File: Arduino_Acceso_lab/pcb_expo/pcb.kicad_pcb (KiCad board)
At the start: 2 copper layers, 88.4 x 55.4 mm, 15 parts, among them P1 modulo wifi, P20 CONN_01X02, U1 LM2576

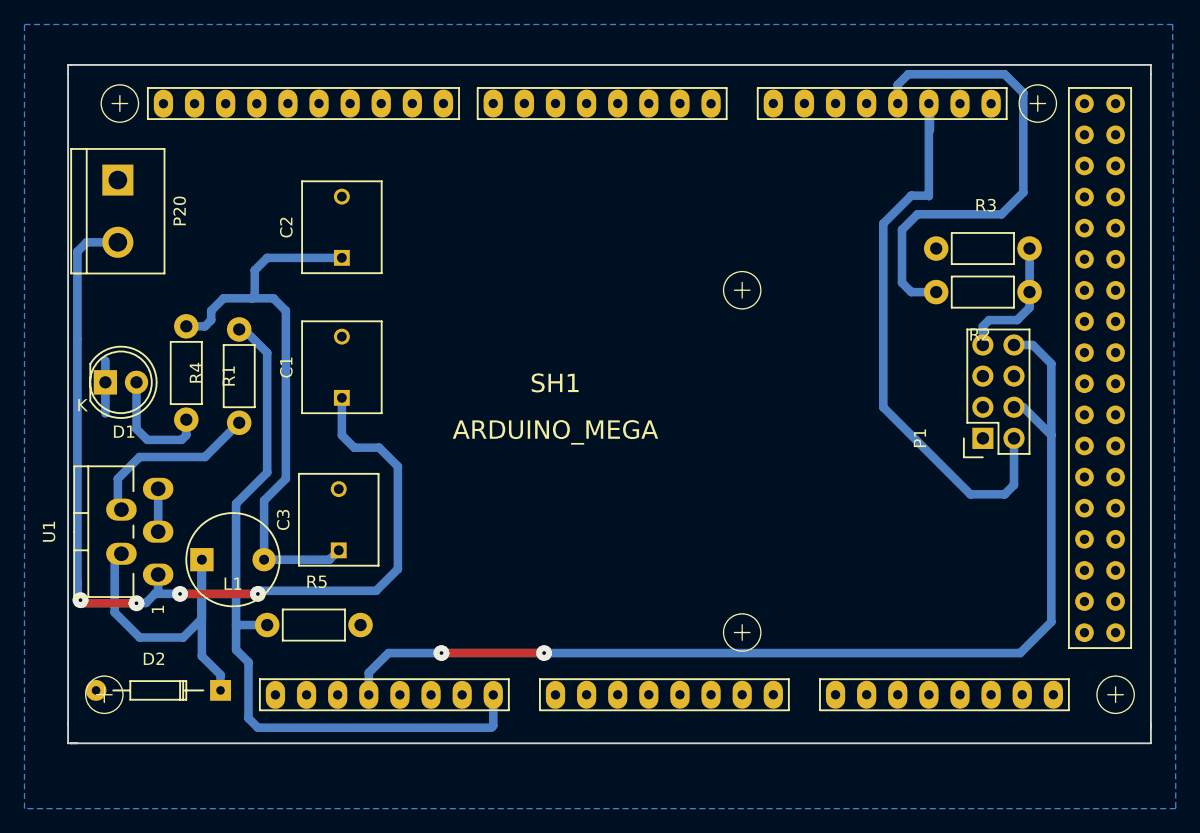
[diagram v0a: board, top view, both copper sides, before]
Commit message: Versión corregida por DJB del Shield Wifi para Arduini Mega.
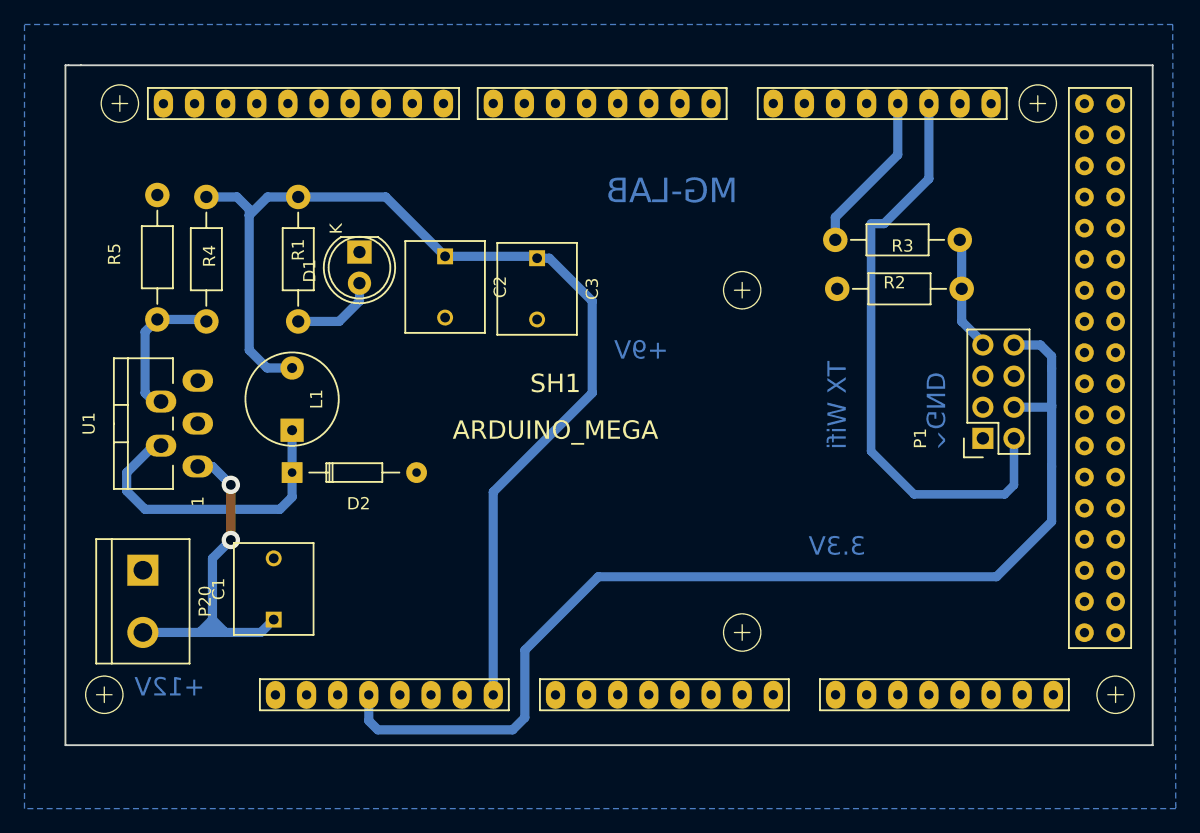
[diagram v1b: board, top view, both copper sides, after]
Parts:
- R1, R2, R3, R4, R5: footprint Resistors_ThroughHole:Resistor_Horizontal_RM7mm -> Resistors_ThroughHole:Resistor_Horizontal_RM10mm
- moved P20 31.9 mm to (114.8, 121.5)
- moved C3 28.8 mm to (147.0, 93.5), turned to 270 degrees
- moved R5 26.5 mm to (116.0, 98.5), turned to 90 degrees
- moved D1 23.3 mm to (132.5, 93.0), turned to 270 degrees
- moved C1 18.9 mm to (125.5, 123.0)
- moved D2 18.7 mm to (127.0, 111.0), turned to 0 degrees
- moved R4 18.6 mm to (120.0, 88.5), turned to 270 degrees
- moved L1 14.0 mm to (127.0, 105.0), turned to 90 degrees
- moved R1 14.0 mm to (127.5, 88.5)
- moved U1 9.40 mm to (115.5, 107.0)
- moved R3 8.72 mm to (171.5, 96.0)
- moved C2 8.43 mm to (139.5, 93.3), turned to 270 degrees
- moved R2 7.12 mm to (181.5, 92.0)
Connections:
- net /3.3 renamed +3.3VP
- C2 pad 1: Net-(C2-Pad1) -> +9V
- C3 pad 1: Net-(C2-Pad1) -> +9V
- L1 pad 2: Net-(C2-Pad1) -> +9V
- P1 pad 2: /RXwifi -> /TXwifi2
- R1 pad 1: Net-(C2-Pad1) -> +9V
- R2 pad 2: /TXwifi -> /RXwifi
- R4 pad 1: Net-(R4-Pad1) -> +9V
- R4 pad 2: +9V -> Net-(R4-Pad2)
- R5 pad 1: +9V -> Net-(R4-Pad2)
- R5 pad 2: Net-(R5-Pad2) -> GND
- SH1 pad 18: /TXwifi -> /RXwifi
- SH1 pad 19: /RXwifi -> /TXwifi2
- U1 pad 3: Net-(U1-Pad3) -> GND
- U1 pad 4: Net-(R4-Pad1) -> Net-(R4-Pad2)
- U1 pad 5: Net-(U1-Pad3) -> GND
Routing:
- net Net-(C1-Pad1): track 78.9 -> 30.3 mm, vias 4 -> 2
- net /TXwifi2: track 0.00 -> 48.3 mm
- net Net-(C2-Pad1): track 47.3 -> 0.00 mm
- net /TXwifi: track 40.0 -> 0.00 mm
- net /RXwifi: track 47.2 -> 13.7 mm
- net +9V: track 60.4 -> 87.7 mm
- net Net-(R4-Pad1): track 14.4 -> 0.00 mm
- net Net-(R4-Pad2): track 0.00 -> 12.1 mm
- net Net-(D2-Pad1): track 29.8 -> 25.2 mm
- net GND: track 4.32 -> 0.00 mm
- net Net-(U1-Pad3): track 3.50 -> 0.00 mm
- net Net-(D1-Pad2): track 9.67 -> 7.15 mm
- net Net-(P1-Pad7): track 10.8 -> 9.37 mm
- net +3.3VP: track 88.0 -> 88.6 mm, vias 2 -> 0
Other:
- board size 88.4 x 55.4 mm -> 88.8 x 55.5 mm
- board text added: "+12V"
- board text added: "+9V"
- board text added: "3.3V"
- board text added: "MG-LAB"
- board text added: "TX Wifi"
- board text added: "^GND"
